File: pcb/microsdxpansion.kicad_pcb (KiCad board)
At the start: 2 copper layers, 32 x 25.5 mm, 8 parts, among them J2 Micro_SD_Card

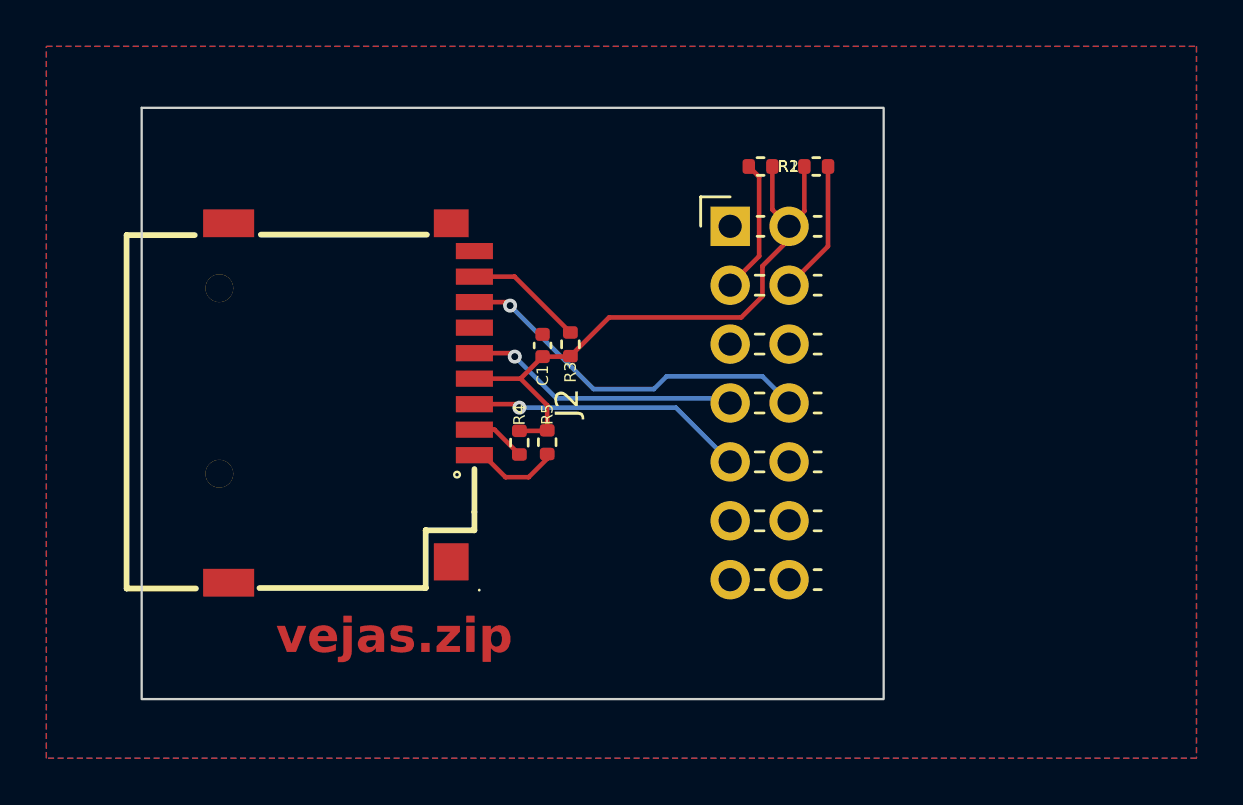
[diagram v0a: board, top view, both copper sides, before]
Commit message: 3d stuff
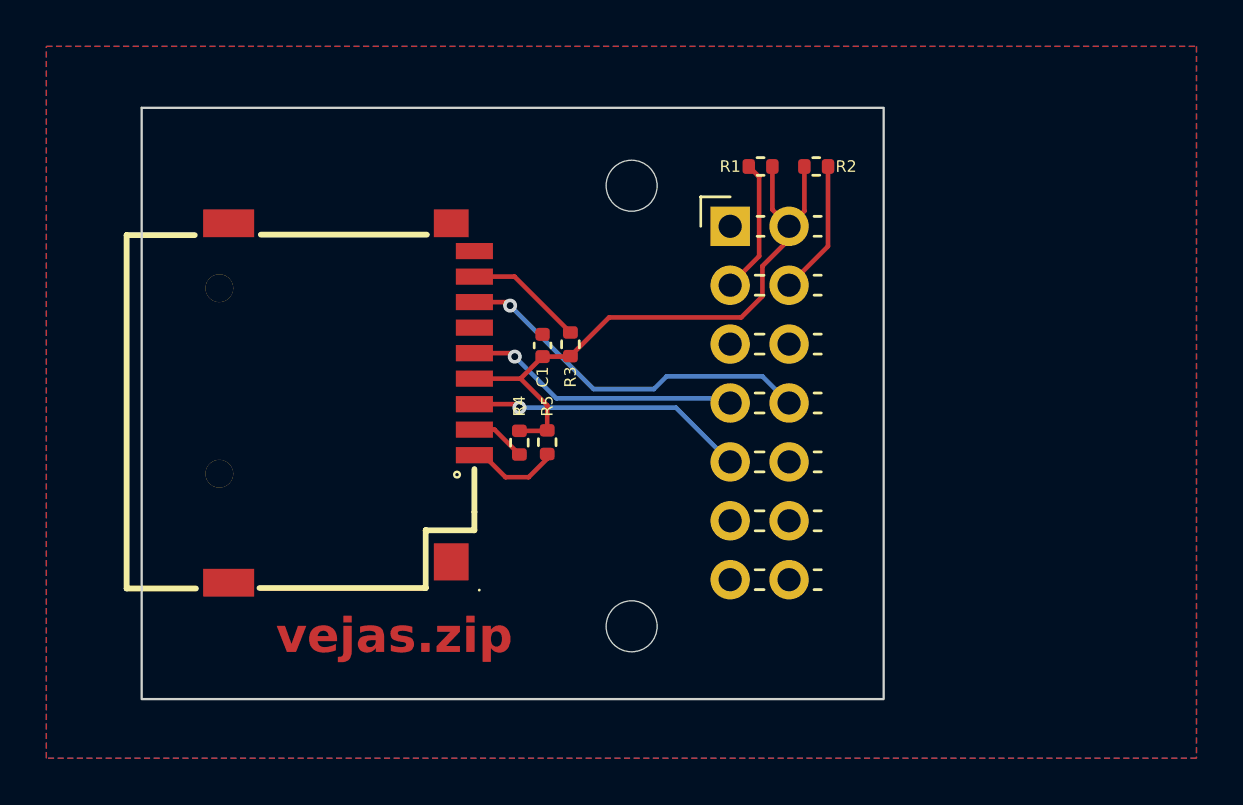
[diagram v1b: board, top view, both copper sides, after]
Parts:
- added REF**: MountingHole_2.2mm_M2, MountingHole:MountingHole_2.2mm_M2, F.Cu at (164.5, 122.0)
- added REF**: MountingHole_2.2mm_M2, MountingHole:MountingHole_2.2mm_M2, F.Cu at (164.5, 103.0)
